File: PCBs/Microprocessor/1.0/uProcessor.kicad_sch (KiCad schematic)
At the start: 109 parts, among them J1 Conn_01x06_Male, J10 Conn_01x02_Male, J11 Conn_01x06_Male, J12 Conn_01x06_Male, J13 Conn_01x02_Male, J14 Conn_01x02_Male, J15 Conn_01x02_Male, J16 Conn_01x02_Male, J17 Conn_01x02_Male, J18 Conn_01x02_Male, J19 Conn_01x02_Male, J2 Conn_01x02_Male, J20 Conn_01x02_Male, J22 Conn_01x04_Male, J23 Conn_01x04_Male, J24 Conn_01x06_Male, J25 Conn_01x04_Male, J26 Conn_01x04_Male, J27 Conn_01x02_Male, J28 Conn_01x02_Male, J29 Conn_01x02_Male, J3 Conn_01x05_Male, J4 Conn_01x03_Male, J5 Conn_01x03_Male, J6 Conn_01x03_Male, J7 Conn_01x03_Male, J8 Conn_01x02_Male, J9 Conn_01x02_Male, Q1 2N3055, Q2 2N3055, Q3 2N3055, Q4 2N3055, SW1 SW_Push, U1 TCA9517DR, U2 FT232RL, U3 ESP32-WROOM-32, U4 AMS1117-3.3, U5 TMP100, Y1 Crystal

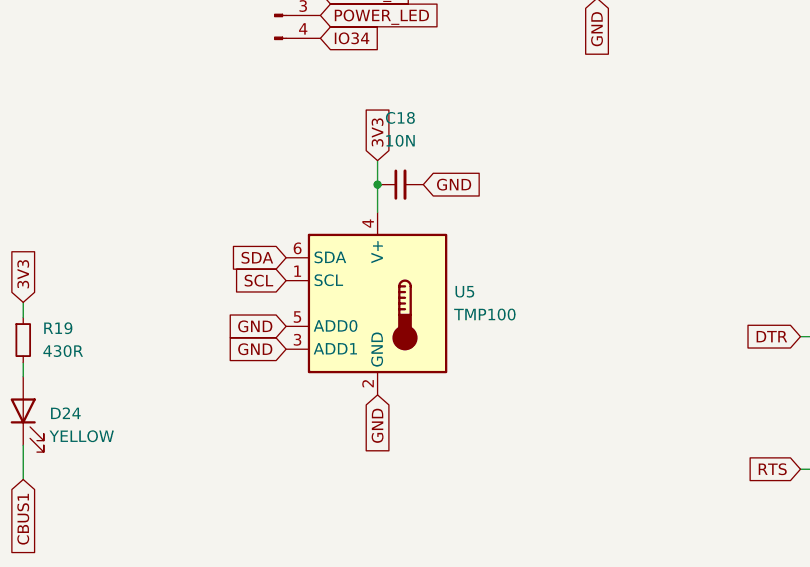
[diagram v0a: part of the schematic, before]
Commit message: Updated
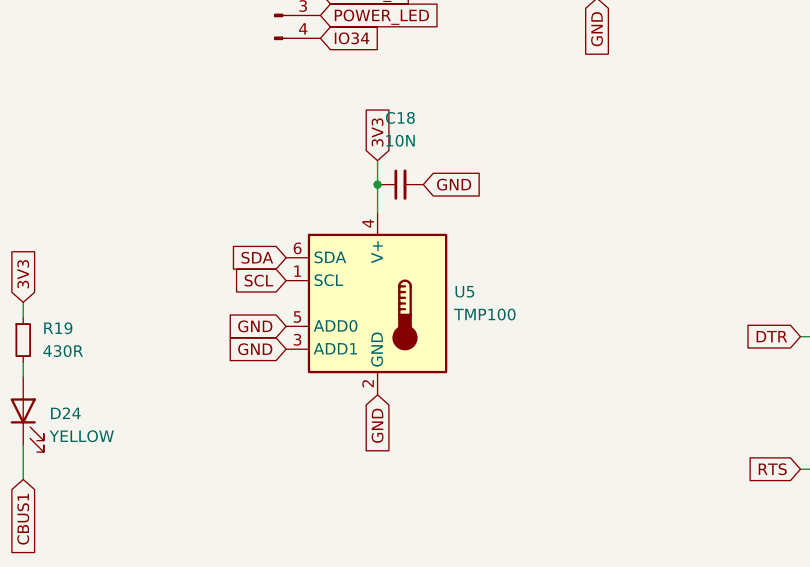
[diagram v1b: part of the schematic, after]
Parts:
- SW1: footprint Button_Switch_SMD:Button_4x4x1.5 -> Components:Button Aliexpress 4x4
